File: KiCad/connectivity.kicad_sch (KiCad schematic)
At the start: 14 parts, among them IC1 NRF7002-QFAA-R7, IC2 SARA-R410M-02B, U17 CXD5610GF, U19 HP5354.A, U21 BGA524N6, U23 BGA524N6, Y3 ECS-TXO-20CSMV4-260-AN-TR

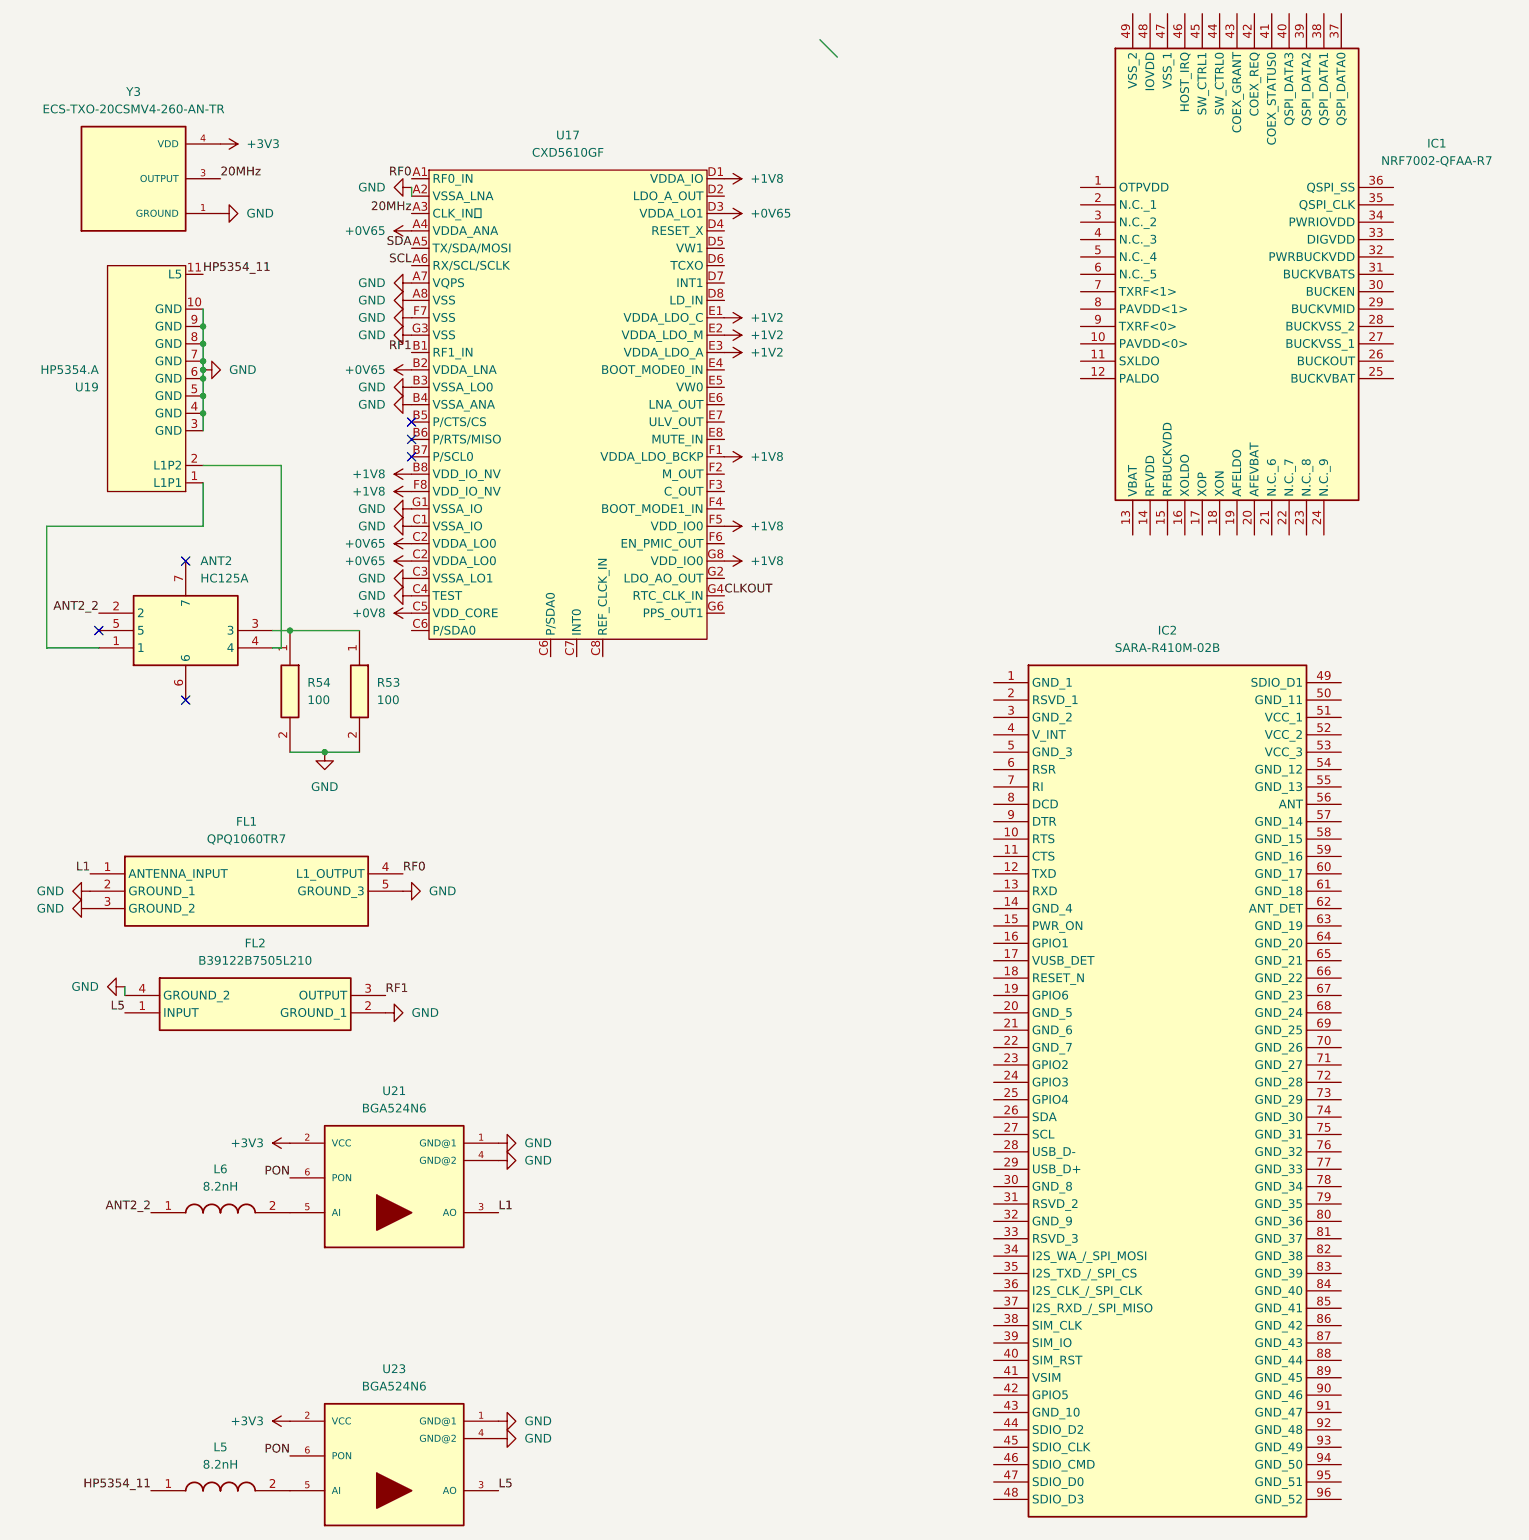
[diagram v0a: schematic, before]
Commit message: simplify
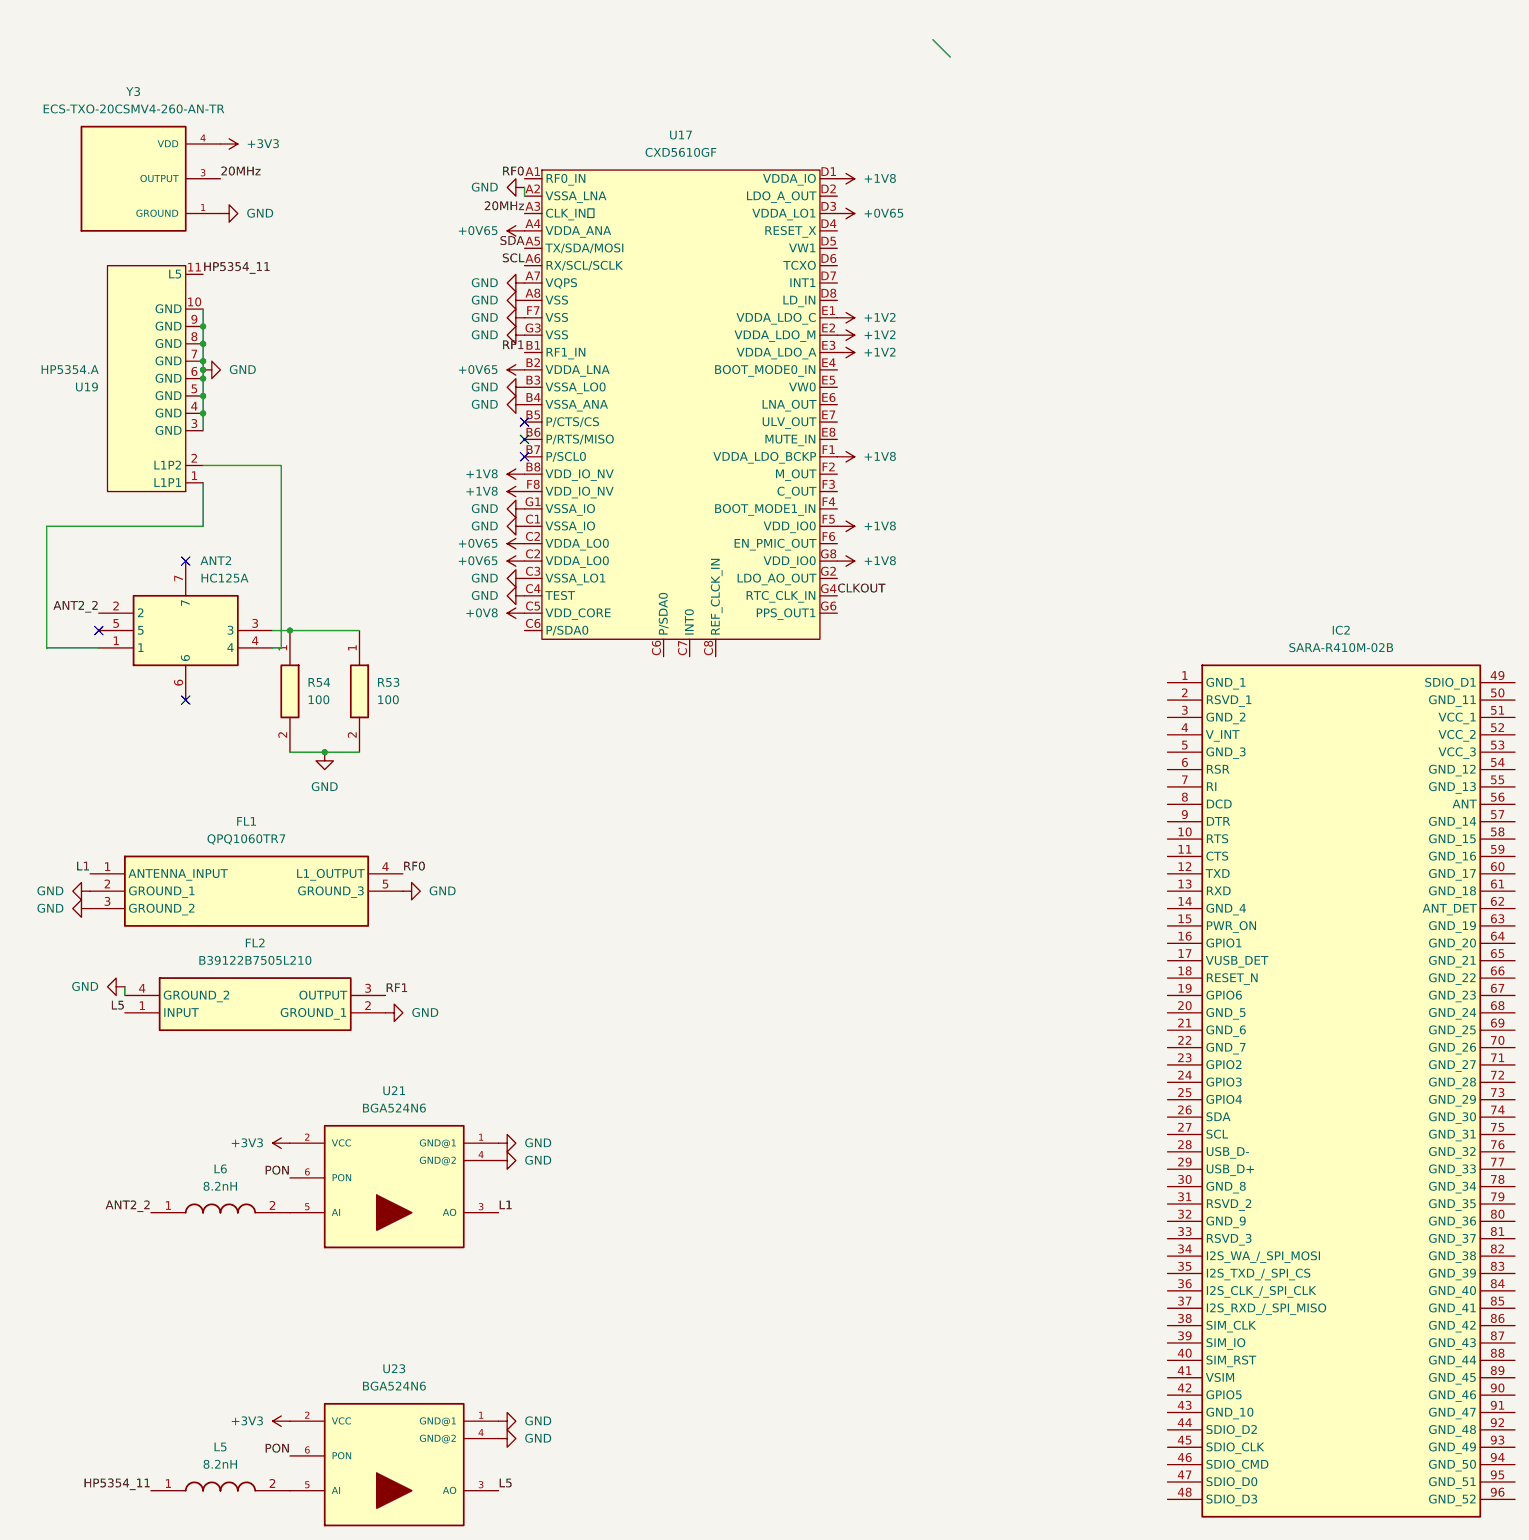
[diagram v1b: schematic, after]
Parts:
- removed IC1: NRF7002-QFAA-R7, QFN40P600X600X95-49N, symbol Symbols:NRF7002-QFAA-R7
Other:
- moved on the sheet: IC2, U17
